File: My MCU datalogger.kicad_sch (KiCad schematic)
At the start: 25 parts, among them U1 24LC1025, U2 DS1307Z, U3 24LC1025, U4 ATMEGA328P-AU, Y1 Crystal, Y2 Crystal

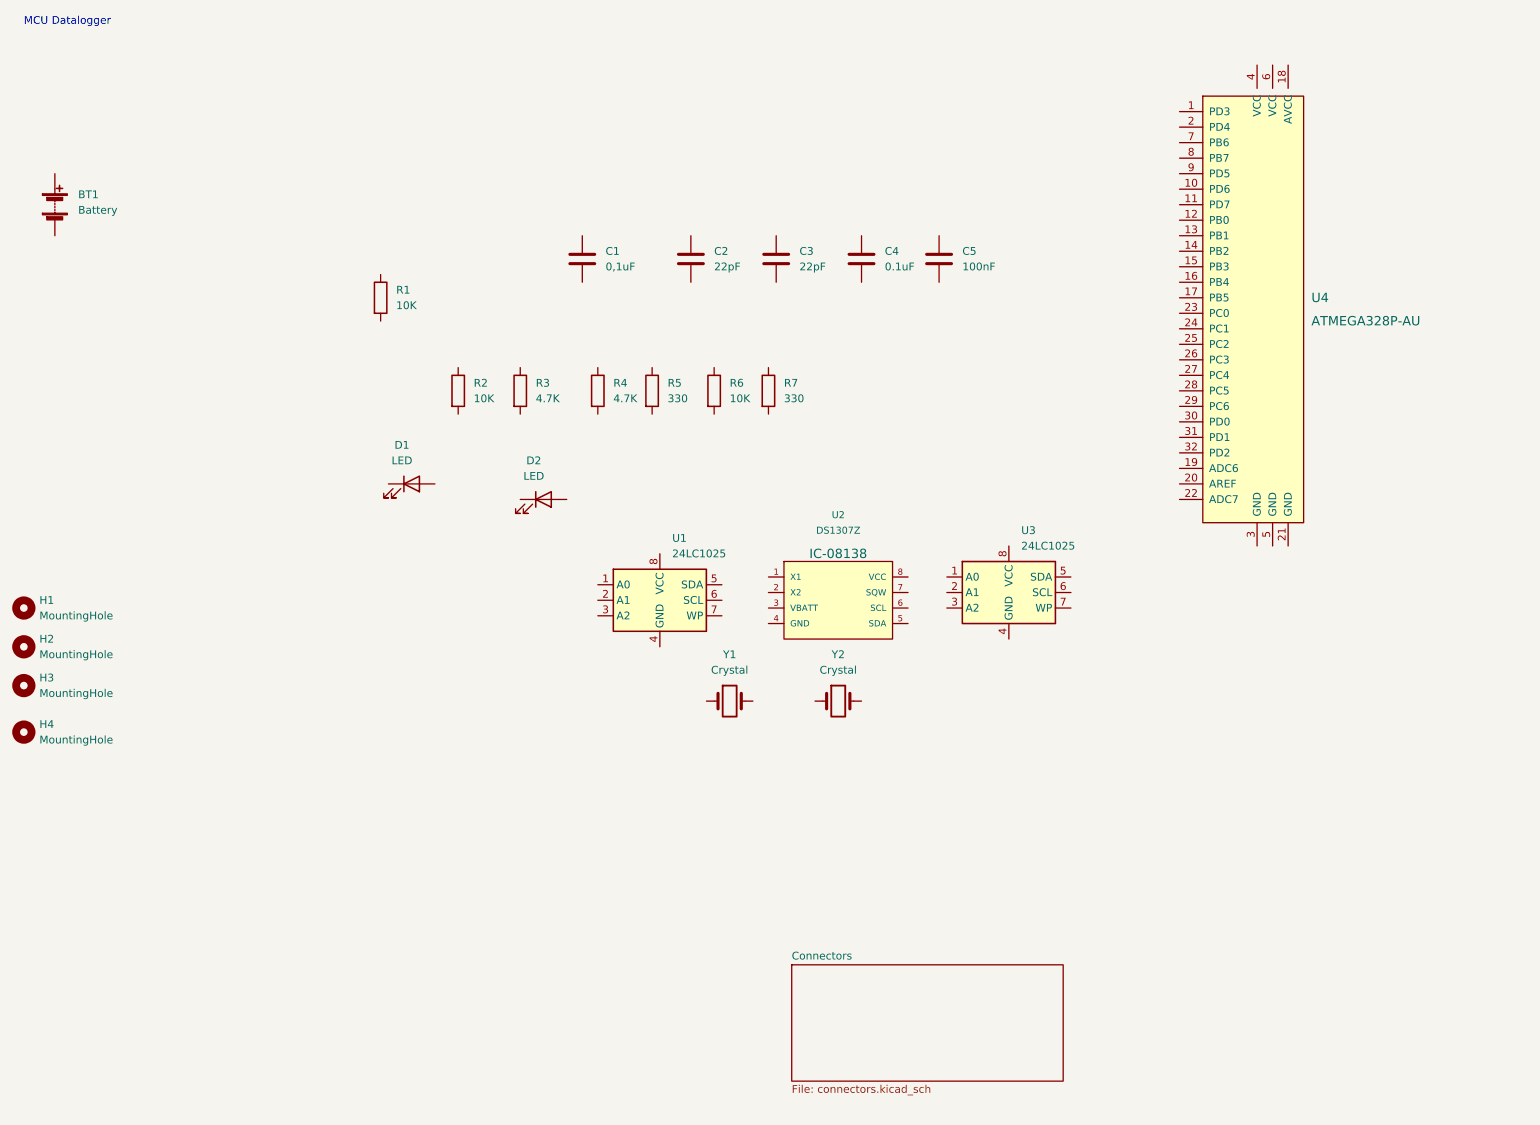
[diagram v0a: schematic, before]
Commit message: Work in progress
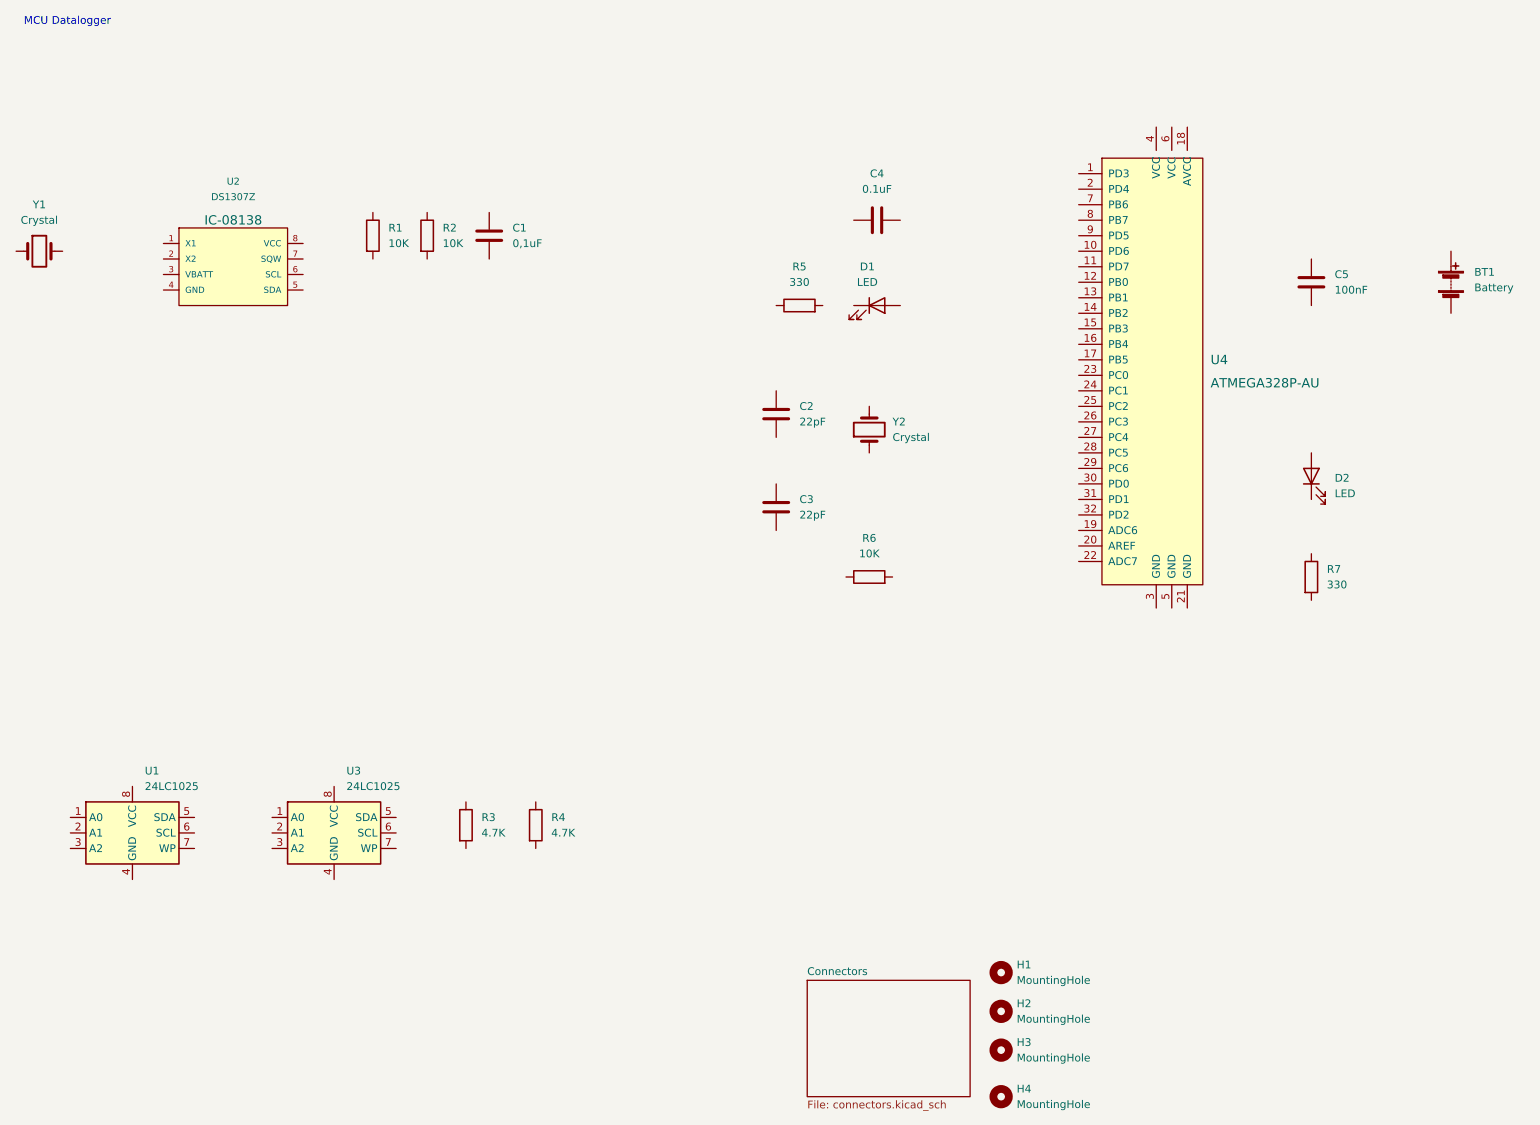
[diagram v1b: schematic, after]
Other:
- moved on the sheet: BT1, C1, C2, C3, C4, C5, D1, D2, H1, H2, H3, H4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
